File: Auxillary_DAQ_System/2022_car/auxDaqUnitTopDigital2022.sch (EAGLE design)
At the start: 44 parts

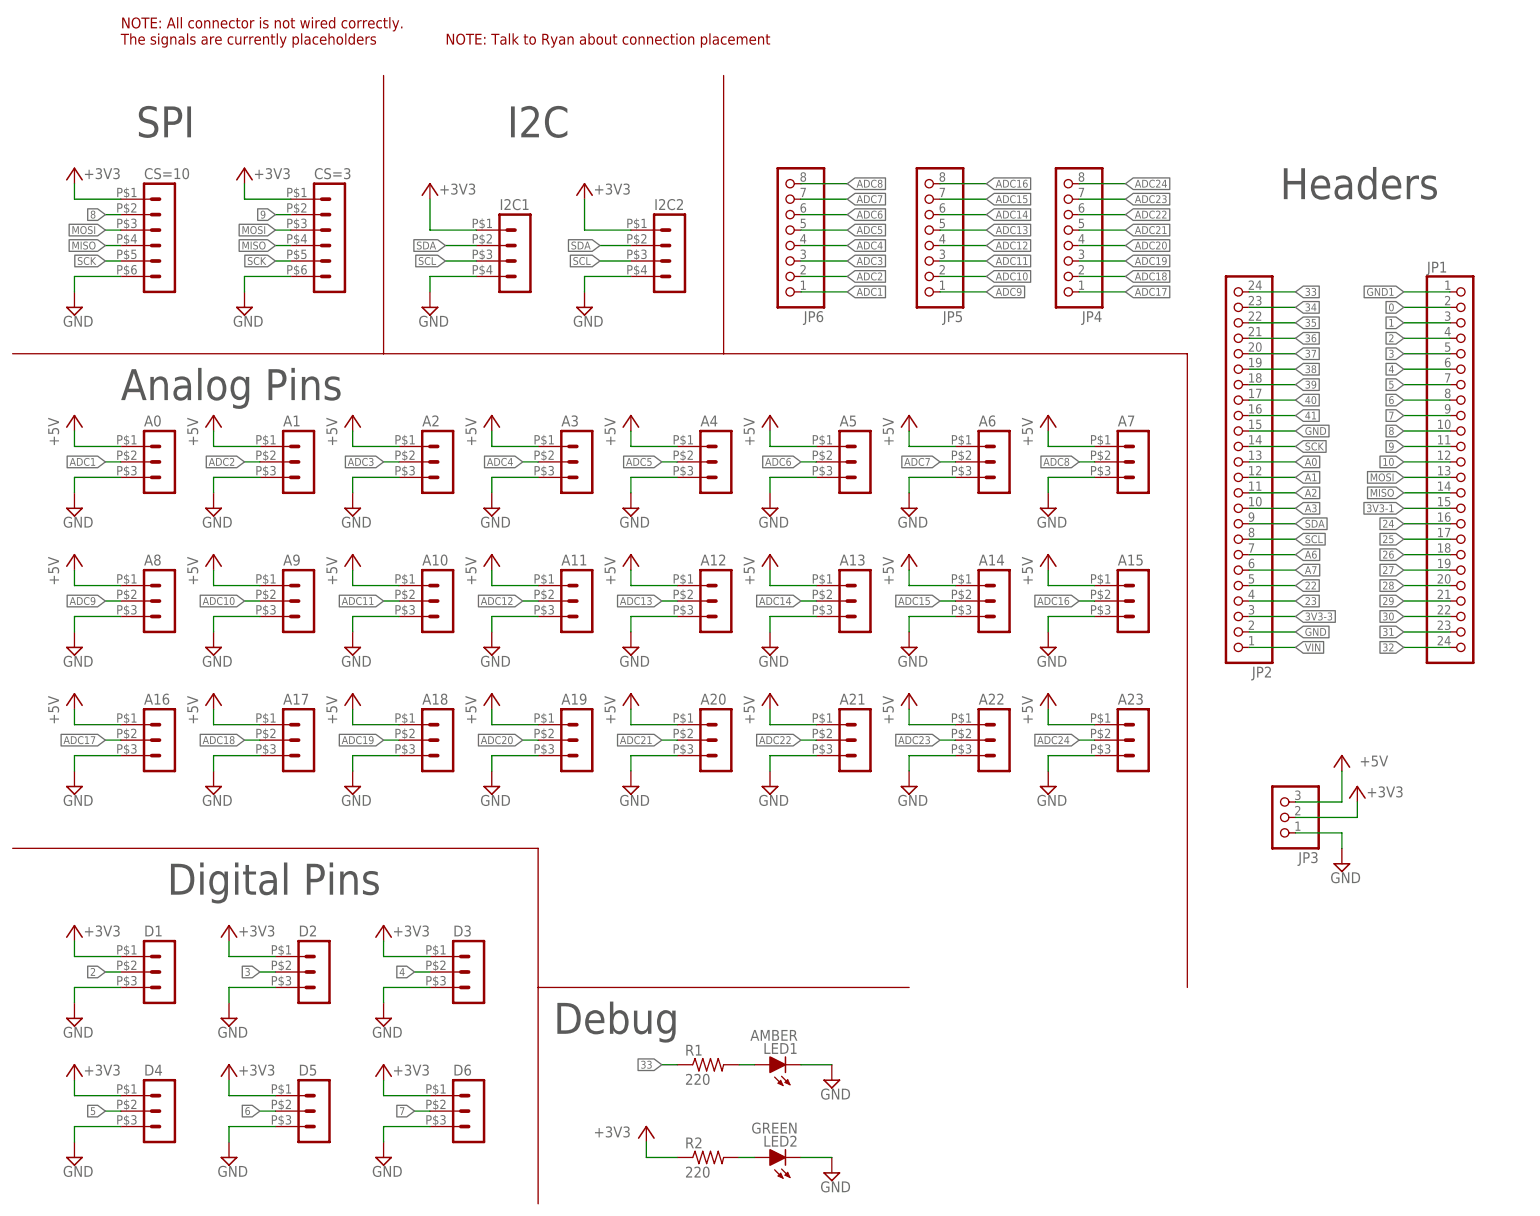
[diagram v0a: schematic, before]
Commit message: Completed auxDAQ rev1
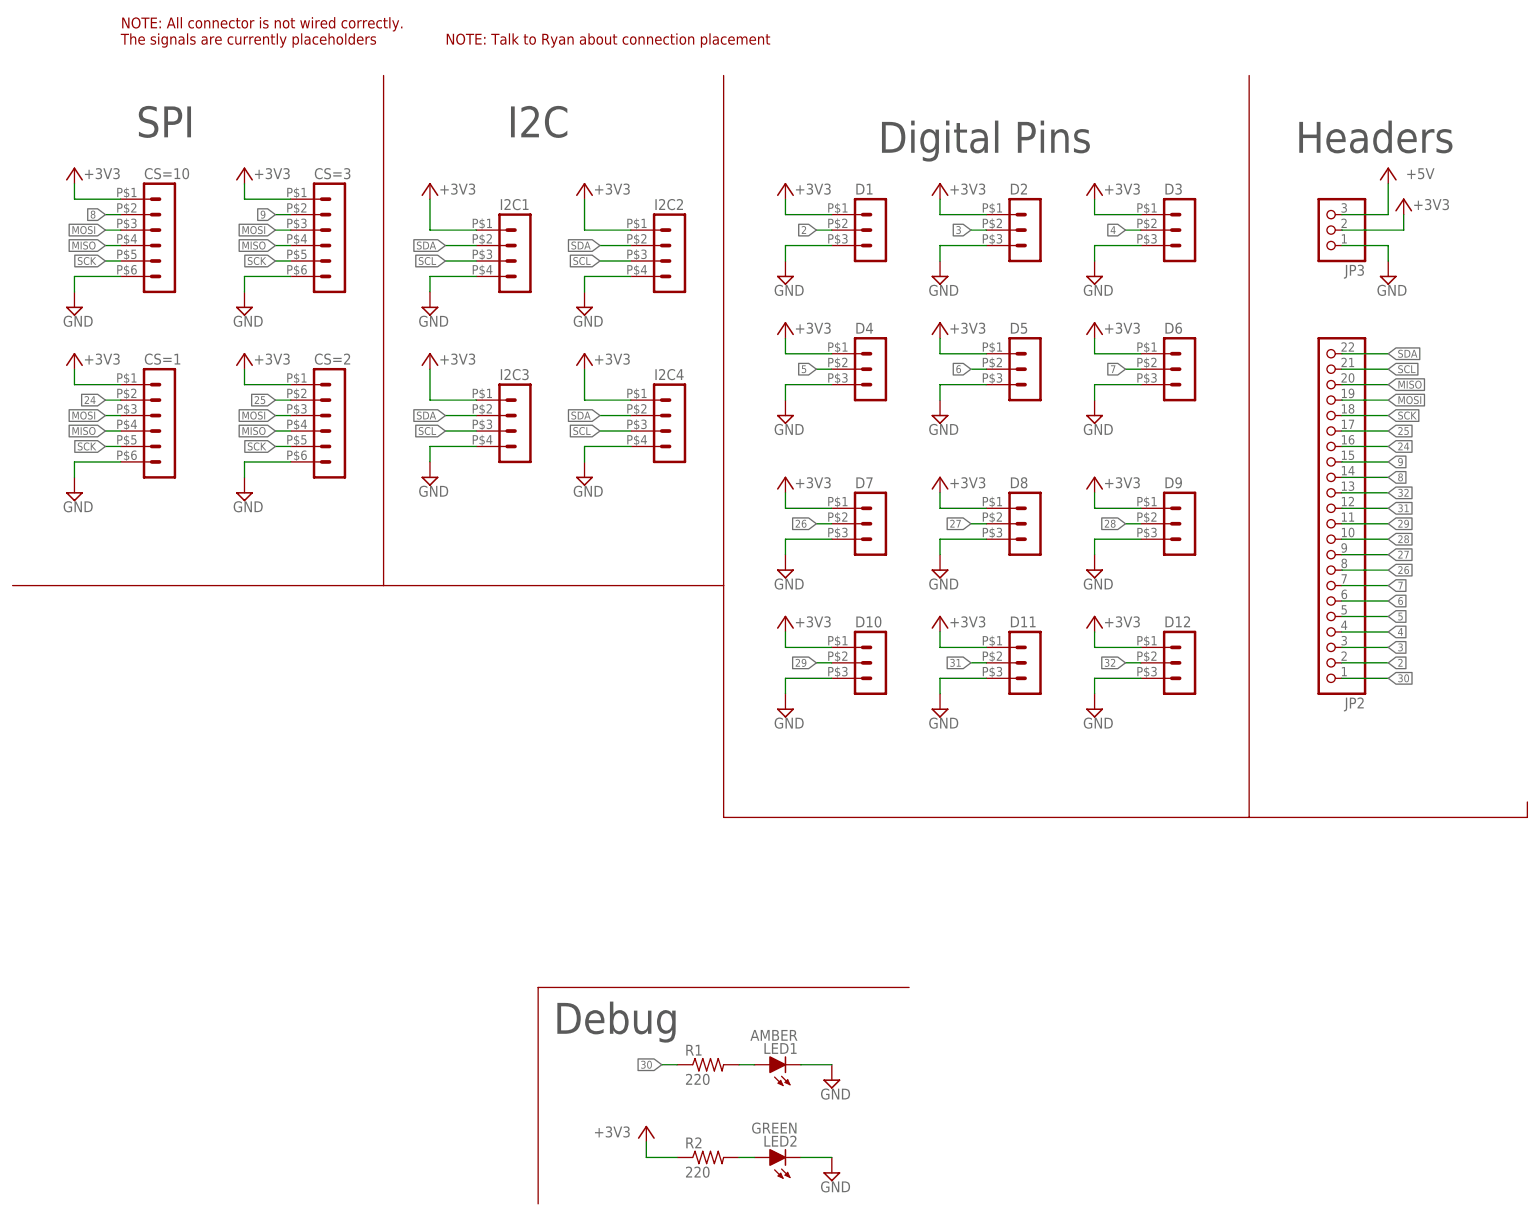
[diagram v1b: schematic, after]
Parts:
- removed A0, A1, A10, A11, A12, A13, A14, A15, A16, A17, A18, A19, A2, A20, A21, A22, A23, A3, A4, A5, A6, A7, A8, A9: (no value), GTOR - Microfit Connector:HEADER_POS3_43650-0300
- removed JP1: (no value), GTOR - Connectors:PINHD-1X24
- removed JP4, JP5, JP6: (no value), GTOR - Connectors:PINHD-1X8
- added CS=1, CS=2: (no value), GTOR - Microfit Connector:HEADER_POS6_43045-0600
- added D10, D11, D12, D7, D8, D9: (no value), GTOR - Microfit Connector:HEADER_POS3_43650-0300
- added I2C3, I2C4: (no value), GTOR - Microfit Connector:HEADER_POS4_43045-0401
- JP2: device GTOR - Connectors:PINHD-1X24 -> GTOR - Connectors:PINHD-1X22
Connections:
- removed net 0: JP1.2
- removed net 1: JP1.3
- removed net 10: JP1.12
- removed net 22: JP2.5
- removed net 23: JP2.4
- removed net 33: JP2.24, R1.1
- removed net 34: JP2.23
- removed net 35: JP2.22
- removed net 36: JP2.21
- removed net 37: JP2.20
- removed net 38: JP2.19
- removed net 39: JP2.18
- removed net 3V3-1: JP1.15
- removed net 3V3-3: JP2.3
- removed net 40: JP2.17
- removed net 41: JP2.16
- removed net A0: JP2.13
- removed net A1: JP2.12
- removed net A2: JP2.11
- removed net A3: JP2.10
- removed net A6: JP2.7
- removed net A7: JP2.6
- removed net ADC1: A0.2, JP6.1
- removed net ADC10: A9.2, JP5.2
- removed net ADC11: A10.2, JP5.3
- removed net ADC12: A11.2, JP5.4
- removed net ADC13: A12.2, JP5.5
- removed net ADC14: A13.2, JP5.6
- removed net ADC15: A14.2, JP5.7
- removed net ADC16: A15.2, JP5.8
- removed net ADC17: A16.2, JP4.1
- removed net ADC18: A17.2, JP4.2
- removed net ADC19: A18.2, JP4.3
- removed net ADC2: A1.2, JP6.2
- removed net ADC20: A19.2, JP4.4
- removed net ADC21: A20.2, JP4.5
- removed net ADC22: A21.2, JP4.6
- removed net ADC23: A22.2, JP4.7
- removed net ADC24: A23.2, JP4.8
- removed net ADC3: A2.2, JP6.3
- removed net ADC4: A3.2, JP6.4
- removed net ADC5: A4.2, JP6.5
- removed net ADC6: A5.2, JP6.6
- removed net ADC7: A6.2, JP6.7
- removed net ADC8: A7.2, JP6.8
- removed net ADC9: A8.2, JP5.1
- removed net GND1: JP1.1
- removed net VIN: JP2.1
- net +3V3: now also CS=1.1, CS=2.1, D10.1, D11.1, D12.1, D7.1, D8.1, D9.1, I2C3.1, I2C4.1
- net +5V: no longer A0.1, A1.1, A10.1, A11.1, A12.1, A13.1, A14.1, A15.1, A16.1, A17.1, A18.1, A19.1, A2.1, A20.1, A21.1, A22.1, A23.1, A3.1, A4.1, A5.1, A6.1, A7.1, A8.1, A9.1
- net 2: now also JP2.2; no longer JP1.4
- net 24: now also CS=1.2, JP2.16; no longer JP1.16
- net 25: now also CS=2.2, JP2.17; no longer JP1.17
- net 26: now also D7.2, JP2.8; no longer JP1.18
- net 27: now also D8.2, JP2.9; no longer JP1.19
- net 28: now also D9.2, JP2.10; no longer JP1.20
- net 29: now also D10.2, JP2.11; no longer JP1.21
- net 3: now also JP2.3; no longer JP1.5
- net 30: now also JP2.1, R1.1; no longer JP1.22
- net 31: now also D11.2, JP2.12; no longer JP1.23
- net 32: now also D12.2, JP2.13; no longer JP1.24
- net 4: now also JP2.4; no longer JP1.6
- net 5: now also JP2.5; no longer JP1.7
- net 6: now also JP2.6; no longer JP1.8
- net 7: now also JP2.7; no longer JP1.9
- net 8: now also JP2.14; no longer JP1.10
- net 9: now also JP2.15; no longer JP1.11
- net GND: now also CS=1.6, CS=2.6, D10.3, D11.3, D12.3, D7.3, D8.3, D9.3, I2C3.4, I2C4.4; no longer A0.3, A1.3, A10.3, A11.3, A12.3, A13.3, A14.3, A15.3, A16.3, A17.3, A18.3, A19.3, A2.3, A20.3, A21.3, A22.3, A23.3, A3.3, A4.3, A5.3, A6.3, A7.3, A8.3, A9.3, JP2.15, JP2.2
- net MISO: now also CS=1.4, CS=2.4, JP2.20; no longer JP1.14
- net MOSI: now also CS=1.3, CS=2.3, JP2.19; no longer JP1.13
- net SCK: now also CS=1.5, CS=2.5, JP2.18; no longer JP2.14
- net SCL: now also I2C3.3, I2C4.3, JP2.21; no longer JP2.8
- net SDA: now also I2C3.2, I2C4.2, JP2.22; no longer JP2.9
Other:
- note removed: "Analog Pins"
- moved on the sheet: D1, D2, D3, D4, D5, D6, JP3
